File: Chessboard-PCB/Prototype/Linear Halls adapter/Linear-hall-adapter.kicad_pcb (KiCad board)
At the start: 2 copper layers, 221 x 101 mm, 37 parts, among them IC1 SS49E, IC10 SS49E, IC11 SS49E, IC12 SS49E, IC13 SS49E, IC14 SS49E, IC15 SS49E, IC16 SS49E, IC17 SS49E, IC18 SS49E, IC19 SS49E, IC2 SS49E, IC20 SS49E, IC21 SS49E, IC22 SS49E, IC23 SS49E, IC24 SS49E, IC25 SS49E, IC26 SS49E, IC27 SS49E, IC28 SS49E, IC29 SS49E, IC3 SS49E, IC30 SS49E, IC31 SS49E, IC32 SS49E, IC4 SS49E, IC5 SS49E, IC6 SS49E, IC7 SS49E, IC8 SS49E, IC9 SS49E, J1 Conn_01x08, J2 Conn_01x02, J3 Conn_01x08, J4 Conn_01x08, J5 Conn_01x08

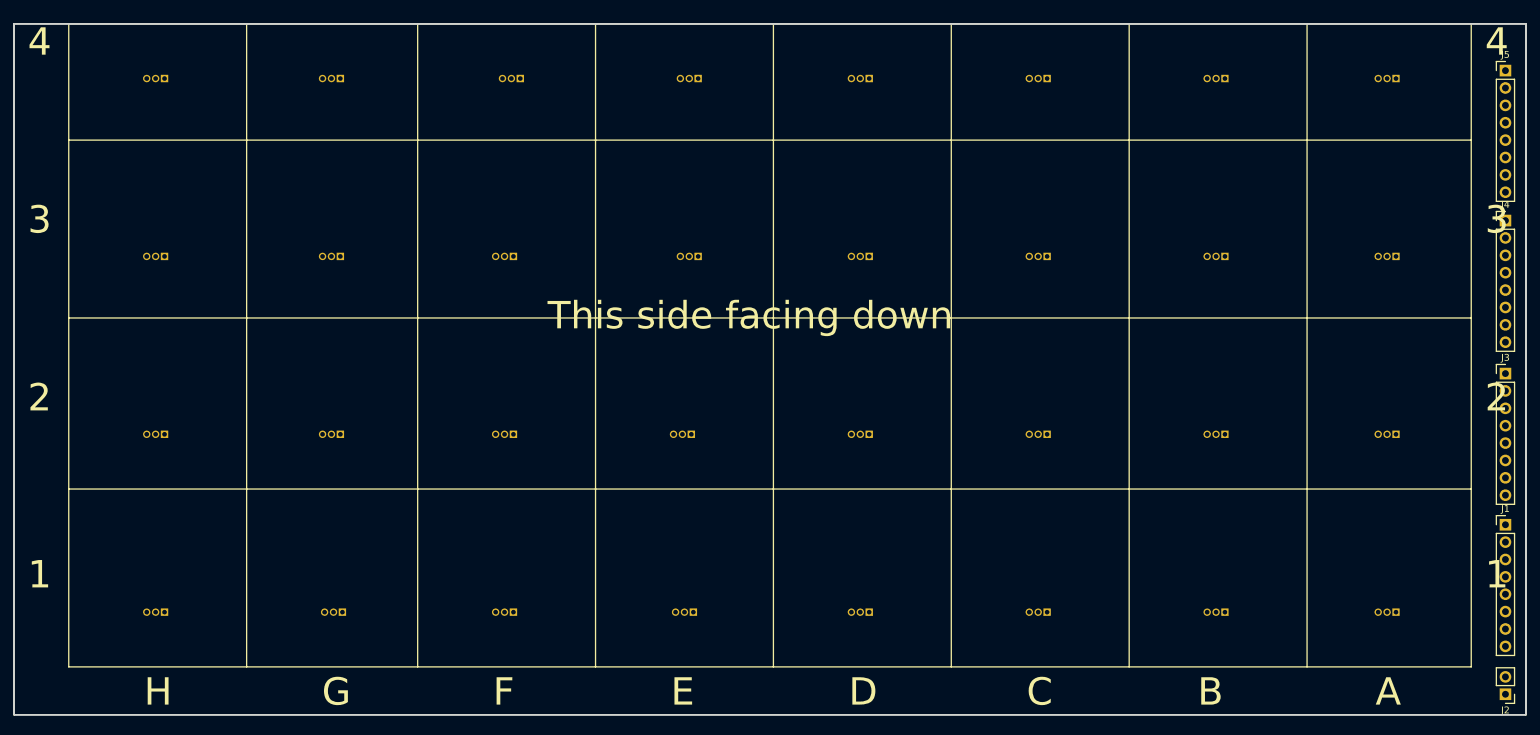
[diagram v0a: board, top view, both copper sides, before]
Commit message: Finish basic PCB
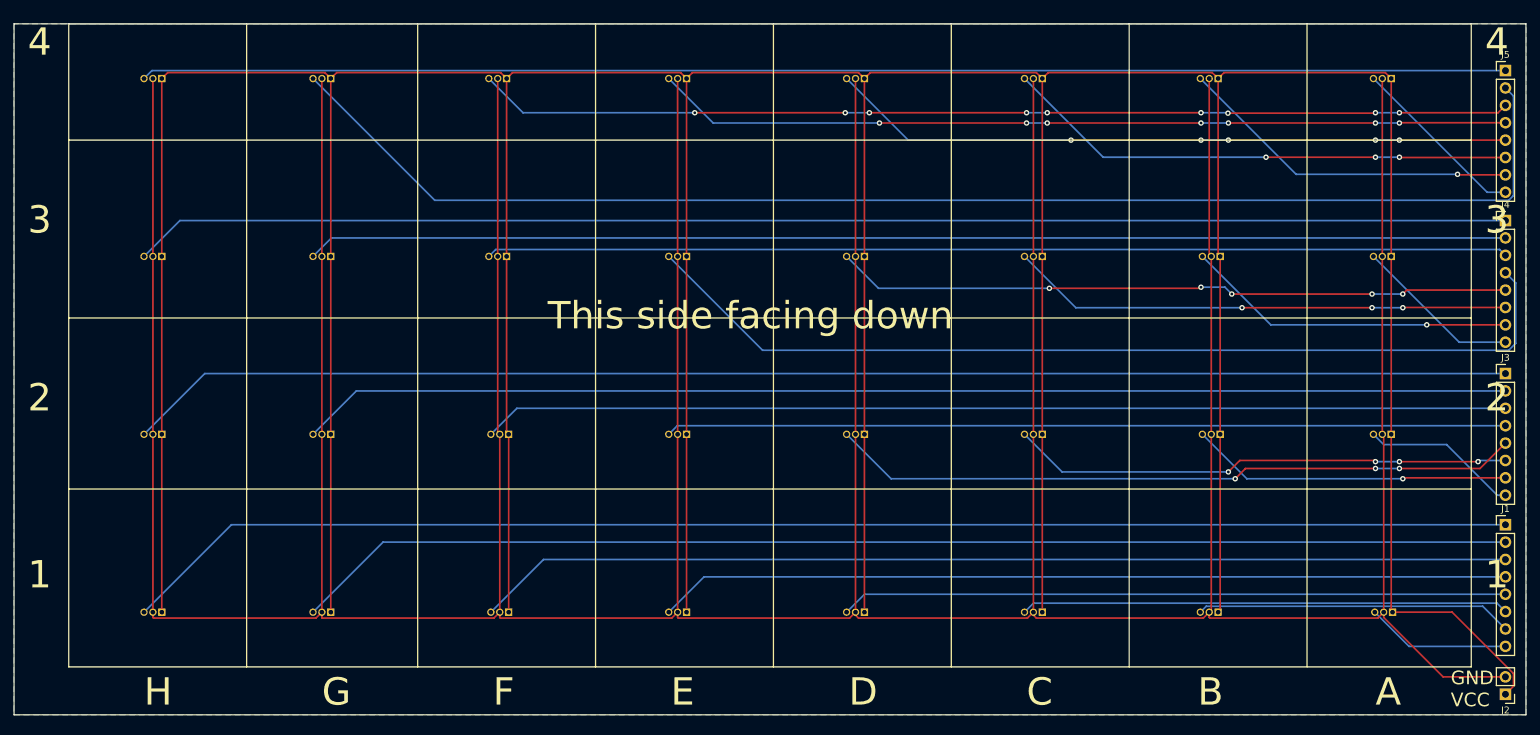
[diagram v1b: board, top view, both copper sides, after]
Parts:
- moved IC27 2.00 mm to (92.0, 28.0)
- moved IC2 1.70 mm to (66.3, 106.0)
- moved IC20 1.70 mm to (118.3, 54.0)
- moved IC28 1.70 mm to (118.3, 28.0)
- moved IC10 1.40 mm to (66.3, 80.0)
- moved IC18 1.40 mm to (66.3, 54.0)
- moved IC26 1.40 mm to (66.3, 28.0)
- moved IC19 1.00 mm to (92.0, 54.0)
- moved IC31 1.00 mm to (196.0, 28.0)
- moved IC4 1.00 mm to (118.3, 106.0)
- moved IC7 1.00 mm to (196.0, 106.0)
- moved IC11 0.70 mm to (92.3, 80.0)
- moved IC12 0.70 mm to (118.3, 80.0)
- moved IC3 0.70 mm to (92.3, 106.0)
- moved IC13 0.70 mm to (144.3, 80.0)
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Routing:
- net VCC: track 0.00 -> 834.5 mm
- net GND: track 0.00 -> 834.3 mm
- net Net-(IC1-O): track 0.00 -> 204.3 mm
- net Net-(IC9-O): track 0.00 -> 202.7 mm
- net Net-(IC17-O): track 0.00 -> 201.2 mm
- net Net-(IC25-O): track 0.00 -> 199.5 mm
- net Net-(IC26-O): track 0.00 -> 199.3 mm
- net Net-(IC2-O): track 0.00 -> 178.5 mm
- net Net-(IC10-O): track 0.00 -> 176.9 mm
- net Net-(IC18-O): track 0.00 -> 175.4 mm
- net Net-(IC3-O): track 0.00 -> 151.5 mm
- net Net-(IC27-O): track 0.00 -> 151.2 mm, vias 0 -> 9
- net Net-(IC11-O): track 0.00 -> 149.9 mm
- net Net-(IC19-O): track 0.00 -> 149.4 mm
- net Net-(IC20-O): track 0.00 -> 140.8 mm
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- added copper zone on B.Cu, net GND
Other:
- board text added: "GND VCC"
